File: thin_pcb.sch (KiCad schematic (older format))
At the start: 149 parts, among them J01 Conn_01x02, J02 Conn_01x02, J04 Conn_01x02, J06 Conn_01x02, J07 Conn_01x02, J08 Conn_01x02, J1 USB_B_Micro, J11 Conn_01x03, J12 Conn_01x03, J13 Conn_01x03, J14 Conn_01x03, J15 Conn_01x03, J16 Conn_01x03, J17 Conn_01x03, J18 Conn_01x03, J2 AudioJack4_Ground, J21 Conn_01x07, J22 Conn_01x07, J23 Conn_01x07, J24 Conn_01x07, J25 Conn_01x07, J26 Conn_01x07, J27 Conn_01x07, J28 Conn_01x07, J3 AudioJack4_Ground, J31 Conn_01x07, J32 Conn_01x07, J33 Conn_01x07, J34 Conn_01x07, J35 Conn_01x07, J36 Conn_01x07, J37 Conn_01x07, J38 Conn_01x07, J4 Conn_01x06, J41 Conn_01x04, J42 Conn_01x04, J43 Conn_01x04, J44 Conn_01x04, J45 Conn_01x04, J46 Conn_01x04, J47 Conn_01x04, J48 Conn_01x04, J5 Conn_01x06, J51 Conn_01x01, J52 Conn_01x01, J53 Conn_01x01, J54 Conn_01x01, J55 Conn_01x01, J56 Conn_01x01, J57 Conn_01x01, J58 Conn_01x01, J6 Conn_02x02, J7 Conn_01x02, SW11 SW_Push, SW12 SW_Push, SW13 SW_Push, SW14 SW_Push, SW15 SW_Push, SW21 SW_Push, SW22 SW_Push, SW23 SW_Push, SW24 SW_Push, SW25 SW_Push, SW252 SW_Push, SW31 SW_Push, SW32 SW_Push, SW33 SW_Push, SW34 SW_Push, SW35 SW_Push, SW41 SW_Push, SW42 SW_Push, SW422 SW_Push, SW43 SW_Push, SW44 SW_Push, SW45 SW_Push, SW452 SW_Push, SW51 SW_Push, SW52 SW_Push, SW522 SW_Push, SW53 SW_Push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

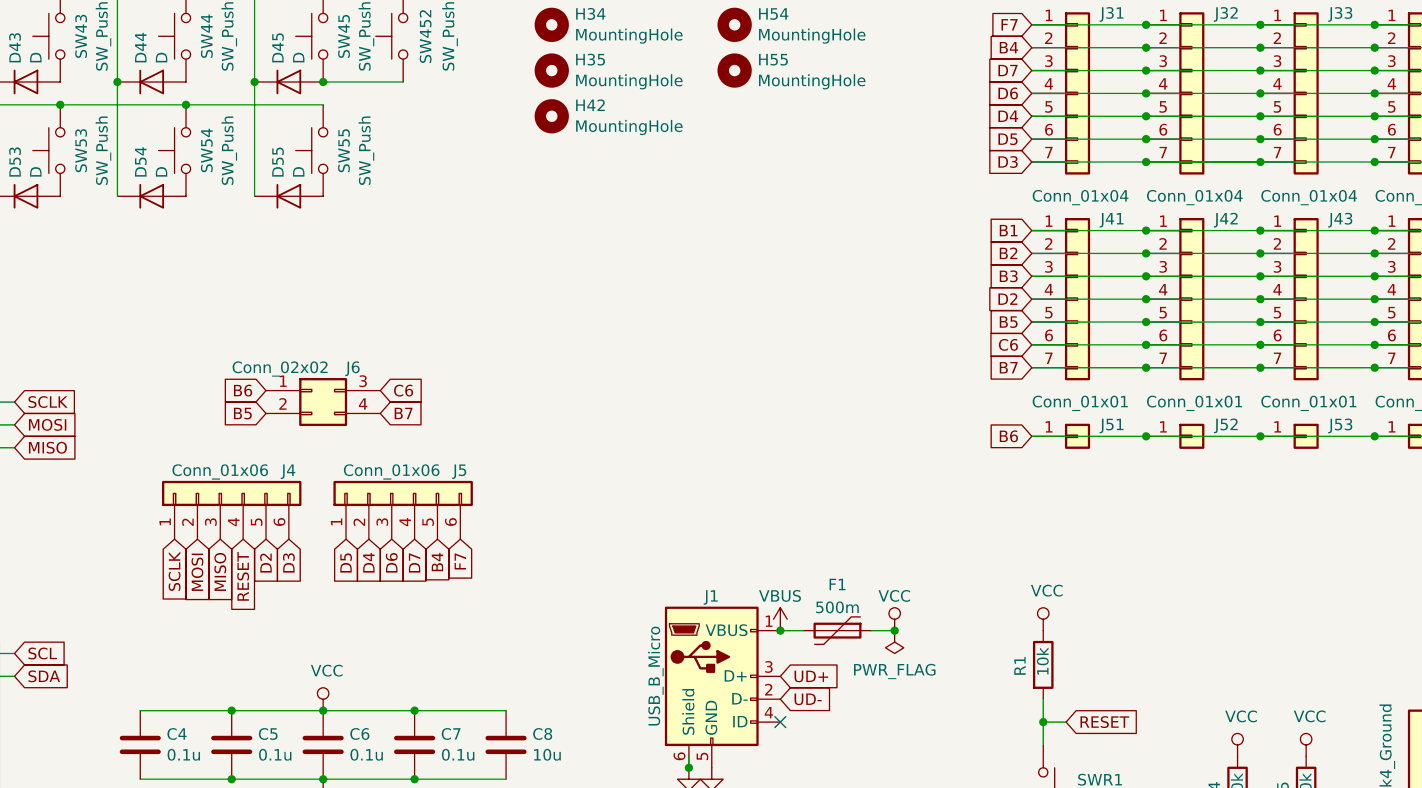
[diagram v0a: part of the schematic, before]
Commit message: reset pinhole
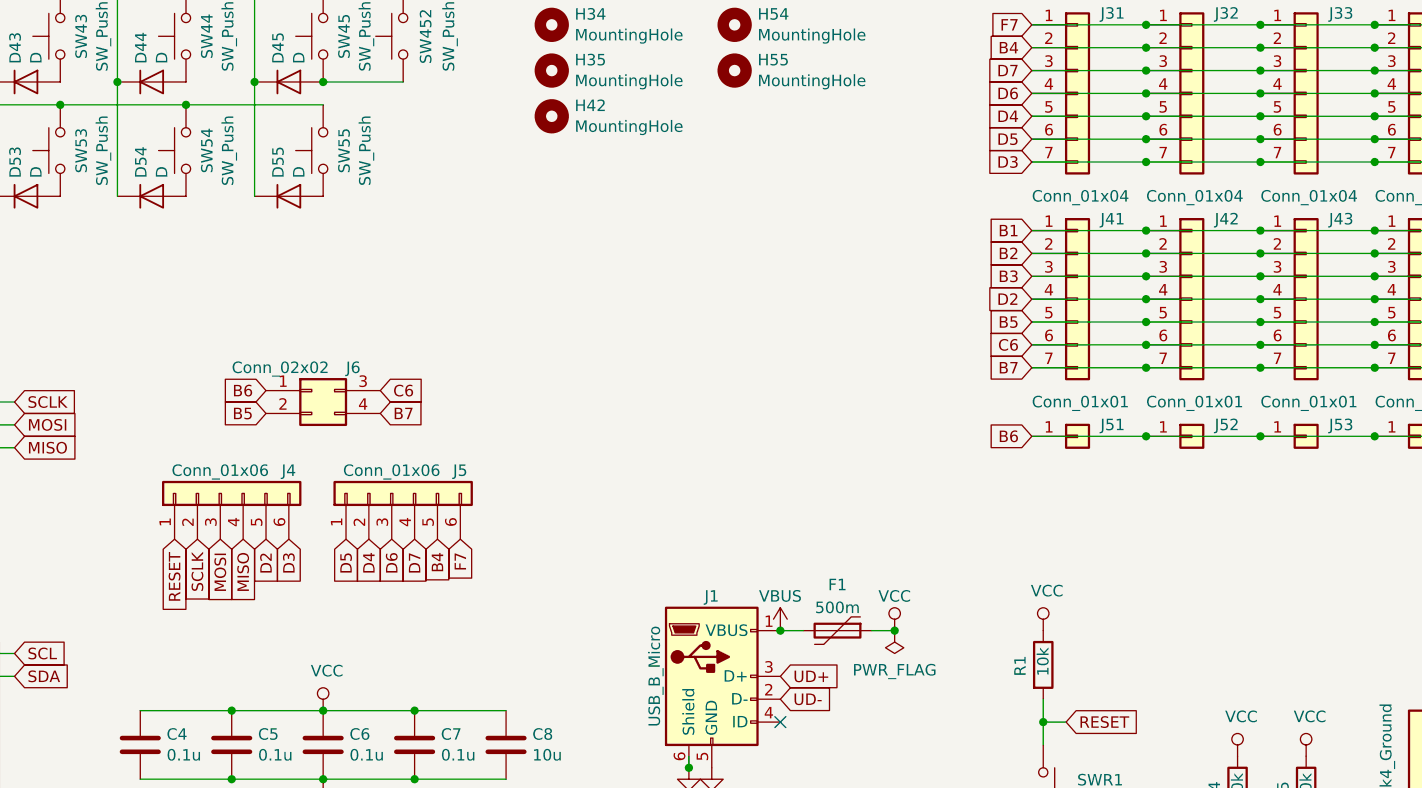
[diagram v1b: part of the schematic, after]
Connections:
- net B1: now also J4.2 (Pin_2); no longer J4.1 (Pin_1)
- net B2: now also J4.3 (Pin_3); no longer J4.2 (Pin_2)
- net B3: now also J4.4 (Pin_4); no longer J4.3 (Pin_3)
- net RESET: now also J4.1 (Pin_1); no longer J4.4 (Pin_4)
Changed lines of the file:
@@
 Text GLabel 9050 5700 2    50   Input ~ 0
 SCL
+Text GLabel 3450 4800 3    50   Input ~ 0
+MISO
 Text GLabel 3350 4800 3    50   Input ~ 0
-MISO
+MOSI
 Text GLabel 3250 4800 3    50   Input ~ 0
-MOSI
+SCLK
 Text GLabel 3150 4800 3    50   Input ~ 0
-SCLK
-Text GLabel 3450 4800 3    50   Input ~ 0
 RESET
 $Comp
@@
 	6900 3050 7400 3050
 Connection ~ 7400 3050
-Wire Wire Line
-	7900 3150 7400 3150
 Connection ~ 7400 3150
 Wire Wire Line

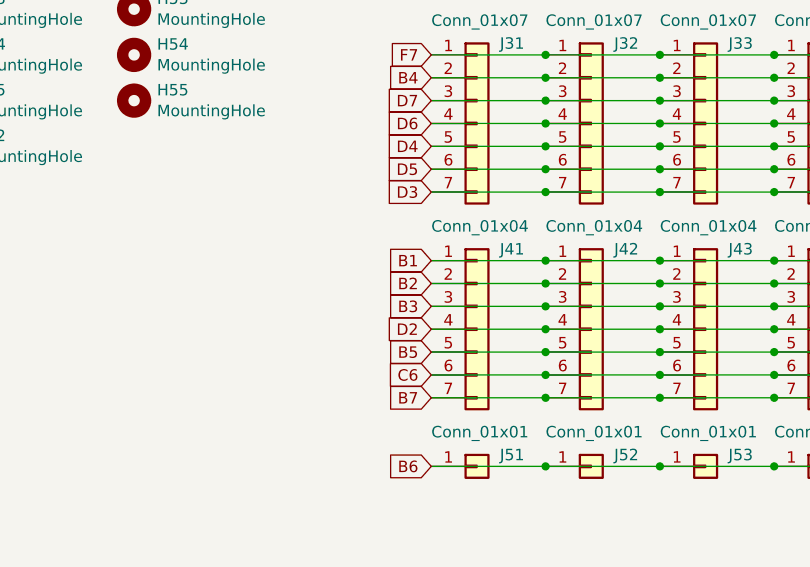
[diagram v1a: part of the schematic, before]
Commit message: breaklines
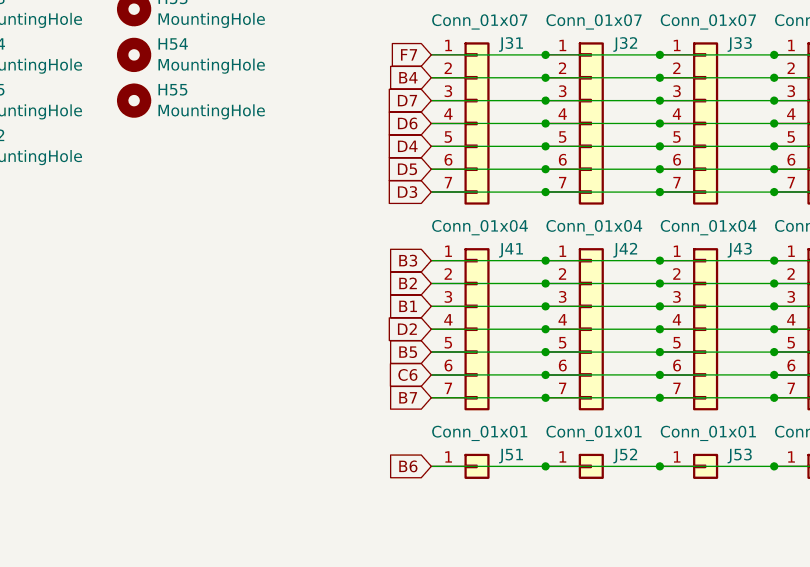
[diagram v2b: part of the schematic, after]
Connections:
- net B1: now also J41.3 (Pin_3), J42.3 (Pin_3), J43.3 (Pin_3), J44.3 (Pin_3), J45.3 (Pin_3), J46.3 (Pin_3), J47.3 (Pin_3), J48.3 (Pin_3); no longer J41.1 (Pin_1), J42.1 (Pin_1), J43.1 (Pin_1), J44.1 (Pin_1), J45.1 (Pin_1), J46.1 (Pin_1), J47.1 (Pin_1), J48.1 (Pin_1)
- net B3: now also J41.1 (Pin_1), J42.1 (Pin_1), J43.1 (Pin_1), J44.1 (Pin_1), J45.1 (Pin_1), J46.1 (Pin_1), J47.1 (Pin_1), J48.1 (Pin_1); no longer J41.3 (Pin_3), J42.3 (Pin_3), J43.3 (Pin_3), J44.3 (Pin_3), J45.3 (Pin_3), J46.3 (Pin_3), J47.3 (Pin_3), J48.3 (Pin_3)
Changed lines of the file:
@@
 Text GLabel 6900 3550 0    50   Input ~ 0
 B2
-Text GLabel 6900 3450 0    50   Input ~ 0
+Text GLabel 6900 3650 0    50   Input ~ 0
 B1
 Text GLabel 6900 3750 0    50   Input ~ 0
@@
 Text GLabel 6900 3050 0    50   Input ~ 0
 D5
-Text GLabel 6900 3650 0    50   Input ~ 0
+Text GLabel 6900 3450 0    50   Input ~ 0
 B3
 Text GLabel 6900 1150 0    50   Input ~ 0
